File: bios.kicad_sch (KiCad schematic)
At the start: 39 parts, among them U12 TMUX1574RSVR, U13 MT25QU01GBBB8_SOIC, U14 TMUX1574RSVR, U15 MT25QU01GBBB8_SOIC

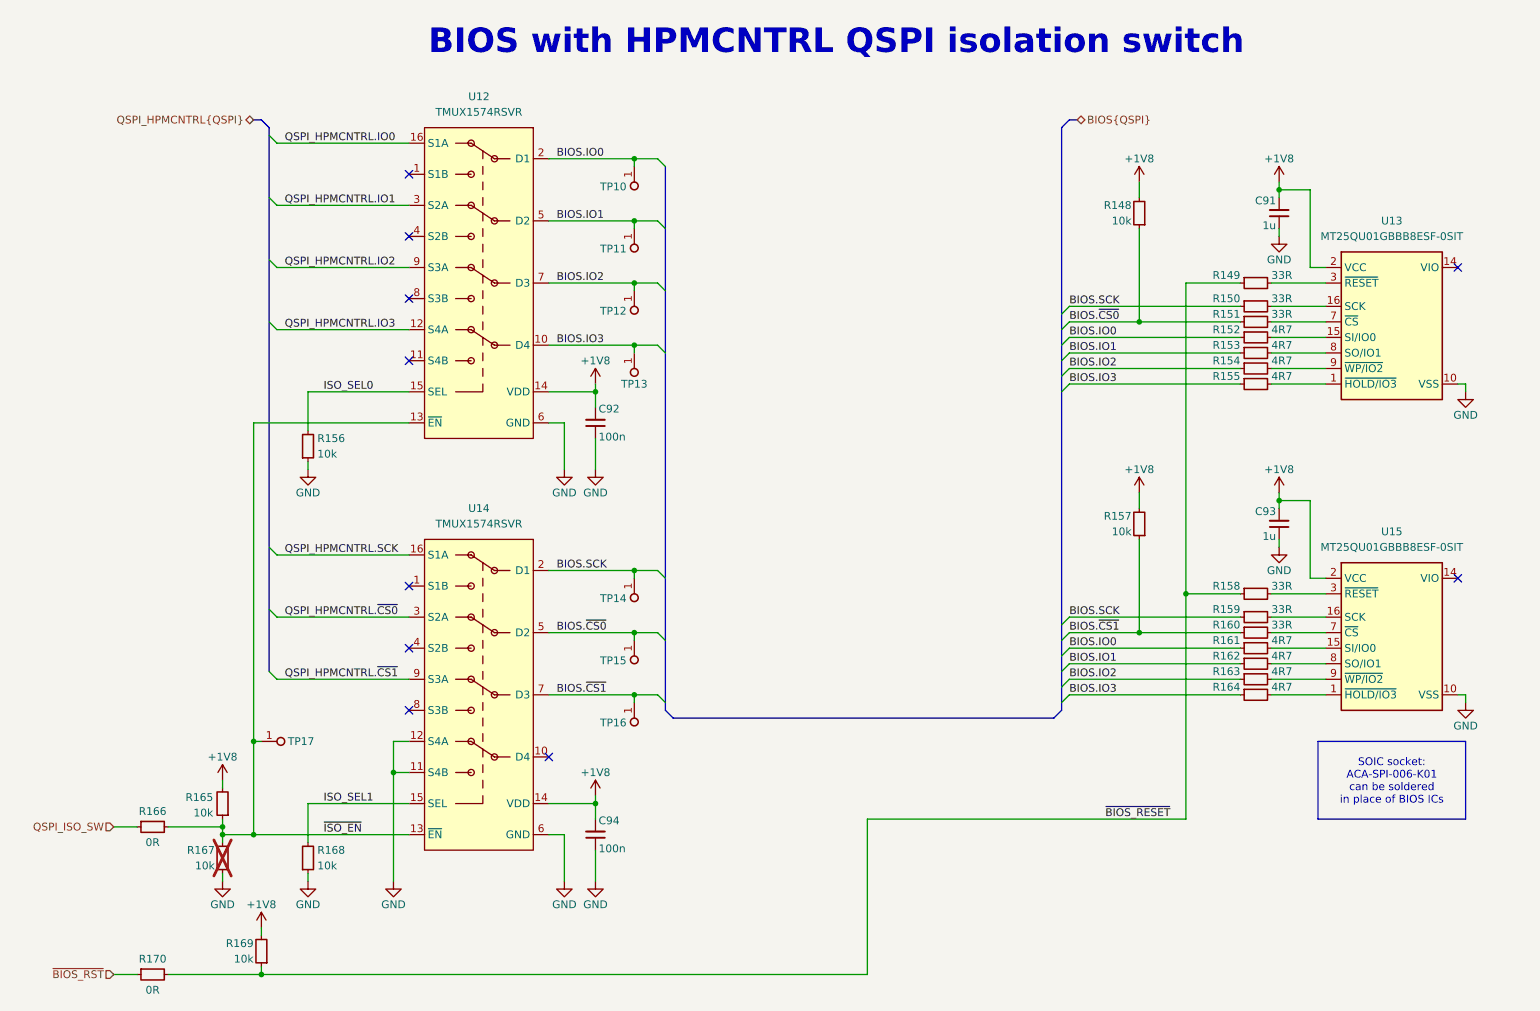
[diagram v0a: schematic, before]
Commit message: [#101340] Add flash sockets
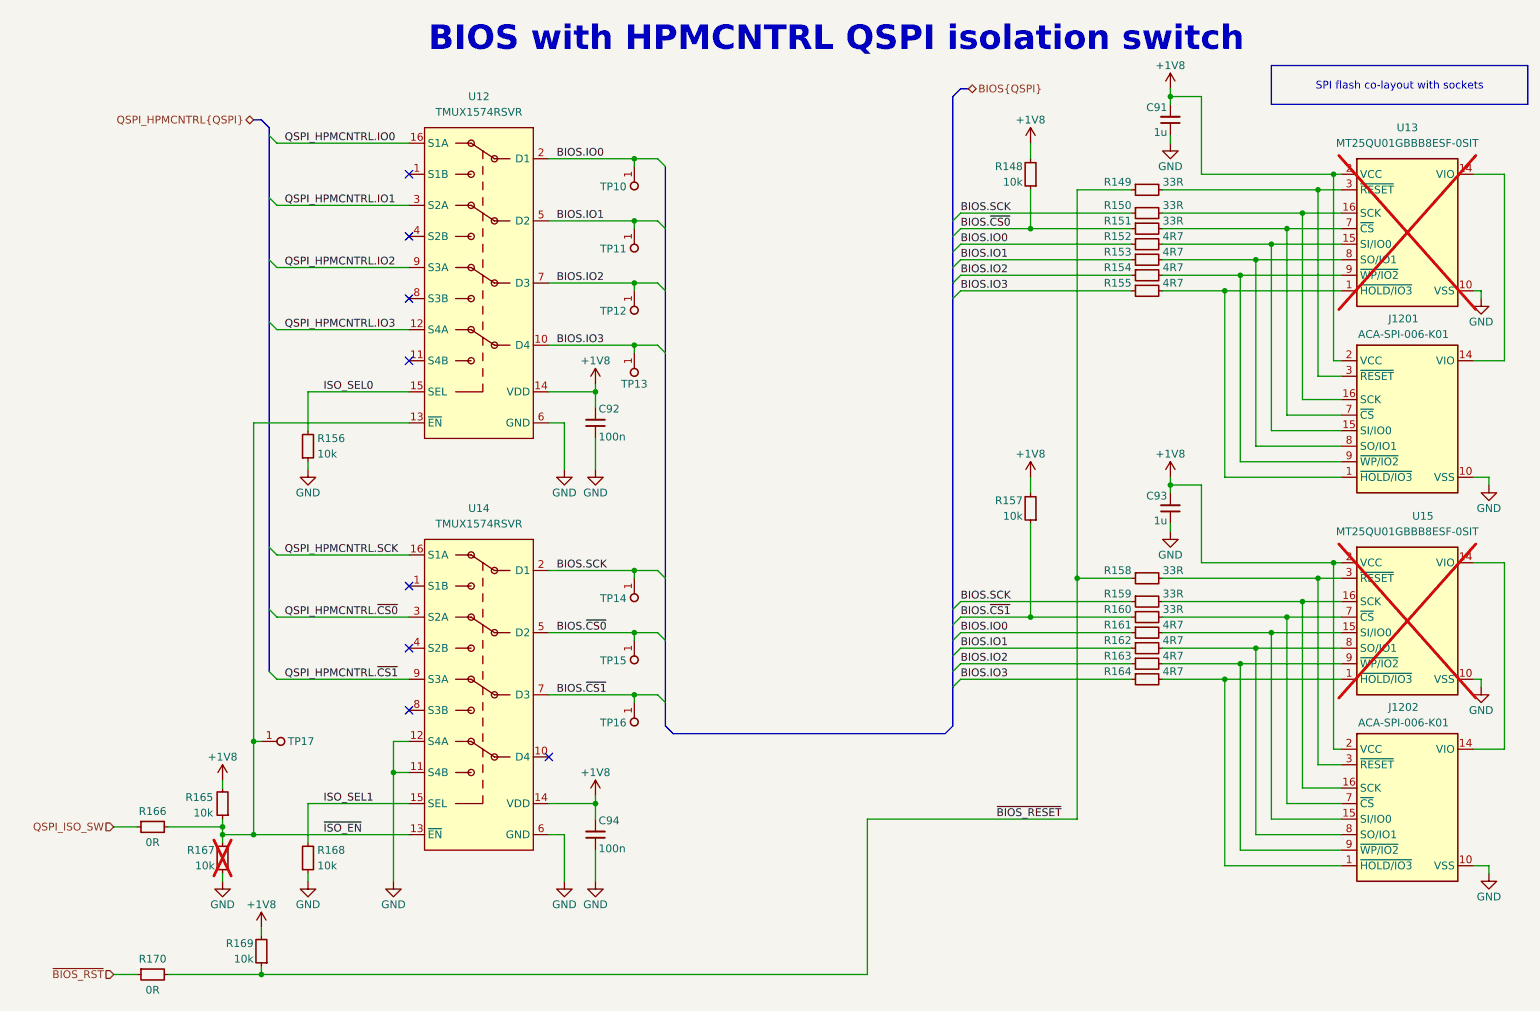
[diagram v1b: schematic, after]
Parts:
- added J1201, J1202: Socket_SOP2-16_ACA-SPI-006-K01_Flash_CUSTOM, antmicro-footprints:Socket_SOP2-16_ACA-SPI-006-K01, symbol antmicroMechanicalParts:Socket_SOP2-16_ACA-SPI-006-K01_Flash_CUSTOM
- U13, U15: now not fitted
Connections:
- net +1V8: now also J1201.2 (VCC), J1202.2 (VCC)
- net GND: now also J1201.10 (VSS), J1202.10 (VSS)
- net at R161.2, U15.15 (SI/IO0): now also J1202.15 (SI/IO0)
- net at R158.2, U15.3 (~{RESET}): now also J1202.3 (~{RESET})
- net at R160.2, U15.7 (~{CS}): now also J1202.7 (~{CS})
- net at R164.2, U15.1 (~{HOLD/IO3}): now also J1202.1 (~{HOLD/IO3})
- net at U15.14 (VIO): now also J1202.14 (VIO)
- net at R159.2, U15.16 (SCK): now also J1202.16 (SCK)
- net at R162.2, U15.8 (SO/IO1): now also J1202.8 (SO/IO1)
- net at R163.2, U15.9 (~{WP/IO2}): now also J1202.9 (~{WP/IO2})
- net at R155.2, U13.1 (~{HOLD/IO3}): now also J1201.1 (~{HOLD/IO3})
- net at U13.14 (VIO): now also J1201.14 (VIO)
- net at R152.2, U13.15 (SI/IO0): now also J1201.15 (SI/IO0)
- net at R150.2, U13.16 (SCK): now also J1201.16 (SCK)
- net at R149.2, U13.3 (~{RESET}): now also J1201.3 (~{RESET})
- net at R151.2, U13.7 (~{CS}): now also J1201.7 (~{CS})
- net at R153.2, U13.8 (SO/IO1): now also J1201.8 (SO/IO1)
- net at R154.2, U13.9 (~{WP/IO2}): now also J1201.9 (~{WP/IO2})
- no-connect marks 10 -> 8
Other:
- moved on the sheet: C91, C93, R148, R149, R150, R151, R152, R153, R154, R155, R157, R158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
